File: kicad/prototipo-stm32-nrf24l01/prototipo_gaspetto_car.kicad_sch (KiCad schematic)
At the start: 11 parts, among them J1 Conn_01x07_Pin - TEST POINT, M1 Motor_DC, M2 Motor_DC, Q1 BC548, U1 YAAJ_BluePill_Part_Like_SWD_B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, U2 nRF24L01+, U3 L9110-M1, U4 L9110-M2

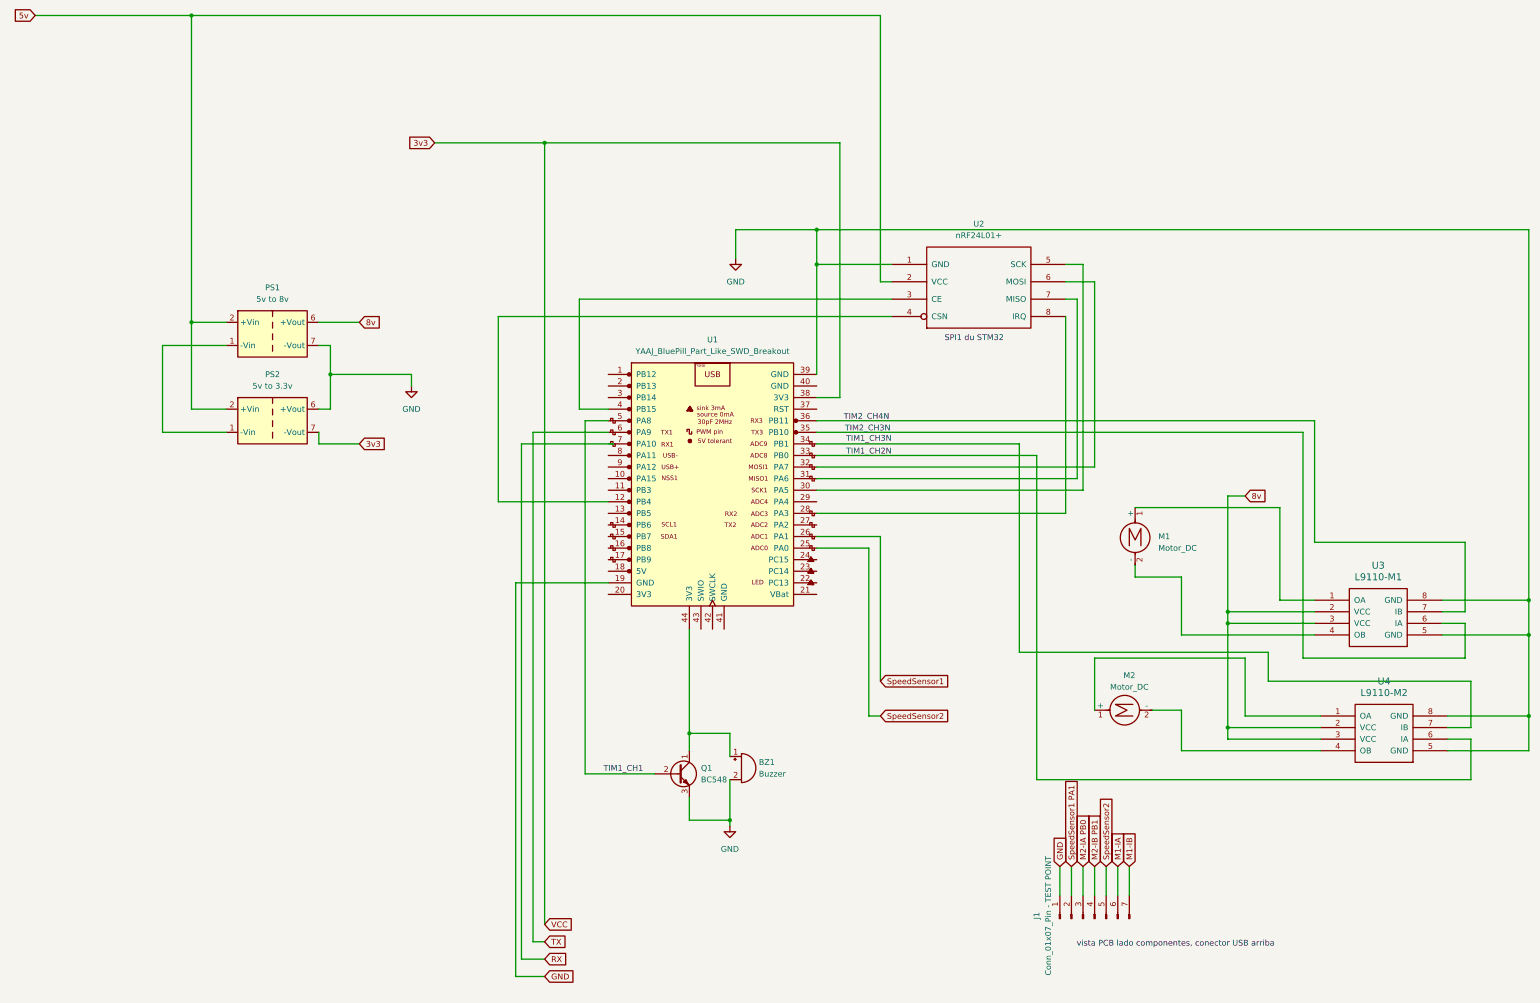
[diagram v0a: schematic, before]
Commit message: kicad: clean projects
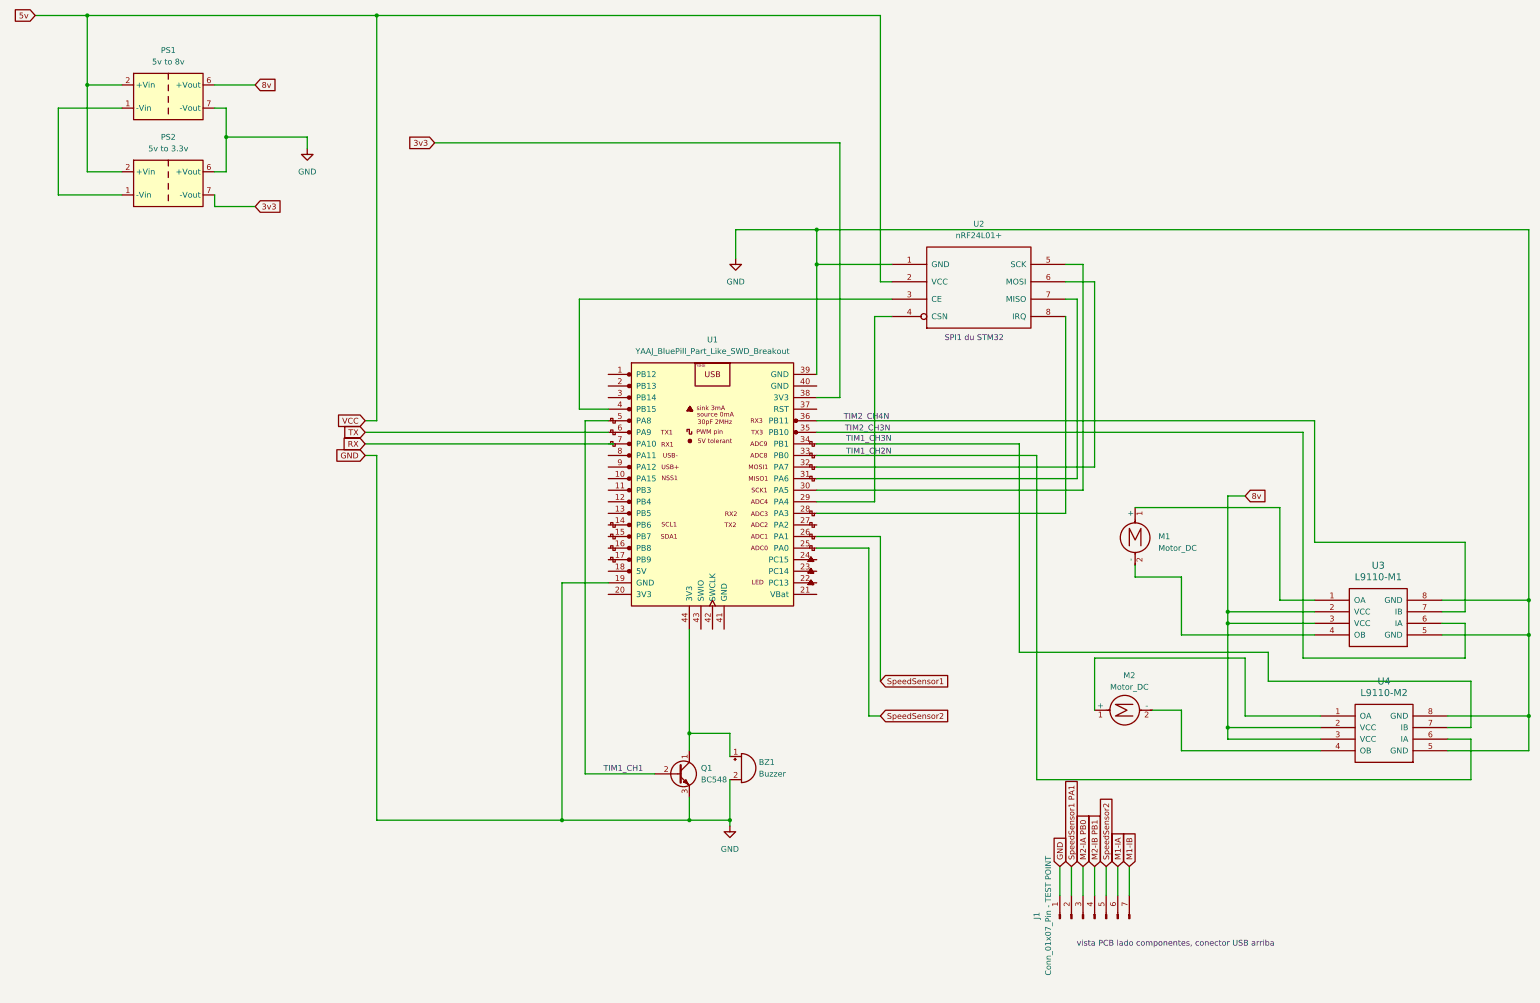
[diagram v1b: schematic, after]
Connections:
- net at U1.12 (PB4): no longer U2.4 (CSN)
- net at U1.29 (PA4): now also U2.4 (CSN)
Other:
- moved on the sheet: PS1, PS2
